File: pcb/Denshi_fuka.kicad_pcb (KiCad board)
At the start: 2 copper layers, 100 x 150 mm, 73 parts, among them J1 Power, J10 JST_PH2P, J11 JST_PH2P, J12 FAN_CONN1, J13 FAN_CONN2, J2 Analog, J3 Digital/PWM, J4 Digital/PWM, J5 SCREW TERMINAL, J6 SCREW TERMINAL, J7 SCREW TERMINAL, J8 SCREW TERMINAL, J9 SCREW TERMINAL, K2 SRD05VDCSLC, Q1 2SC1815, Q2 2SK3176, Q3 2SK3176, U1 Si8651, U10 MCP3564R, U2 LM2940T-3.3, U3 LM358, U4 MCP6232, U5 PS817, U6 PS817, U7 PS817, U8 PS817, U9 MCP4822

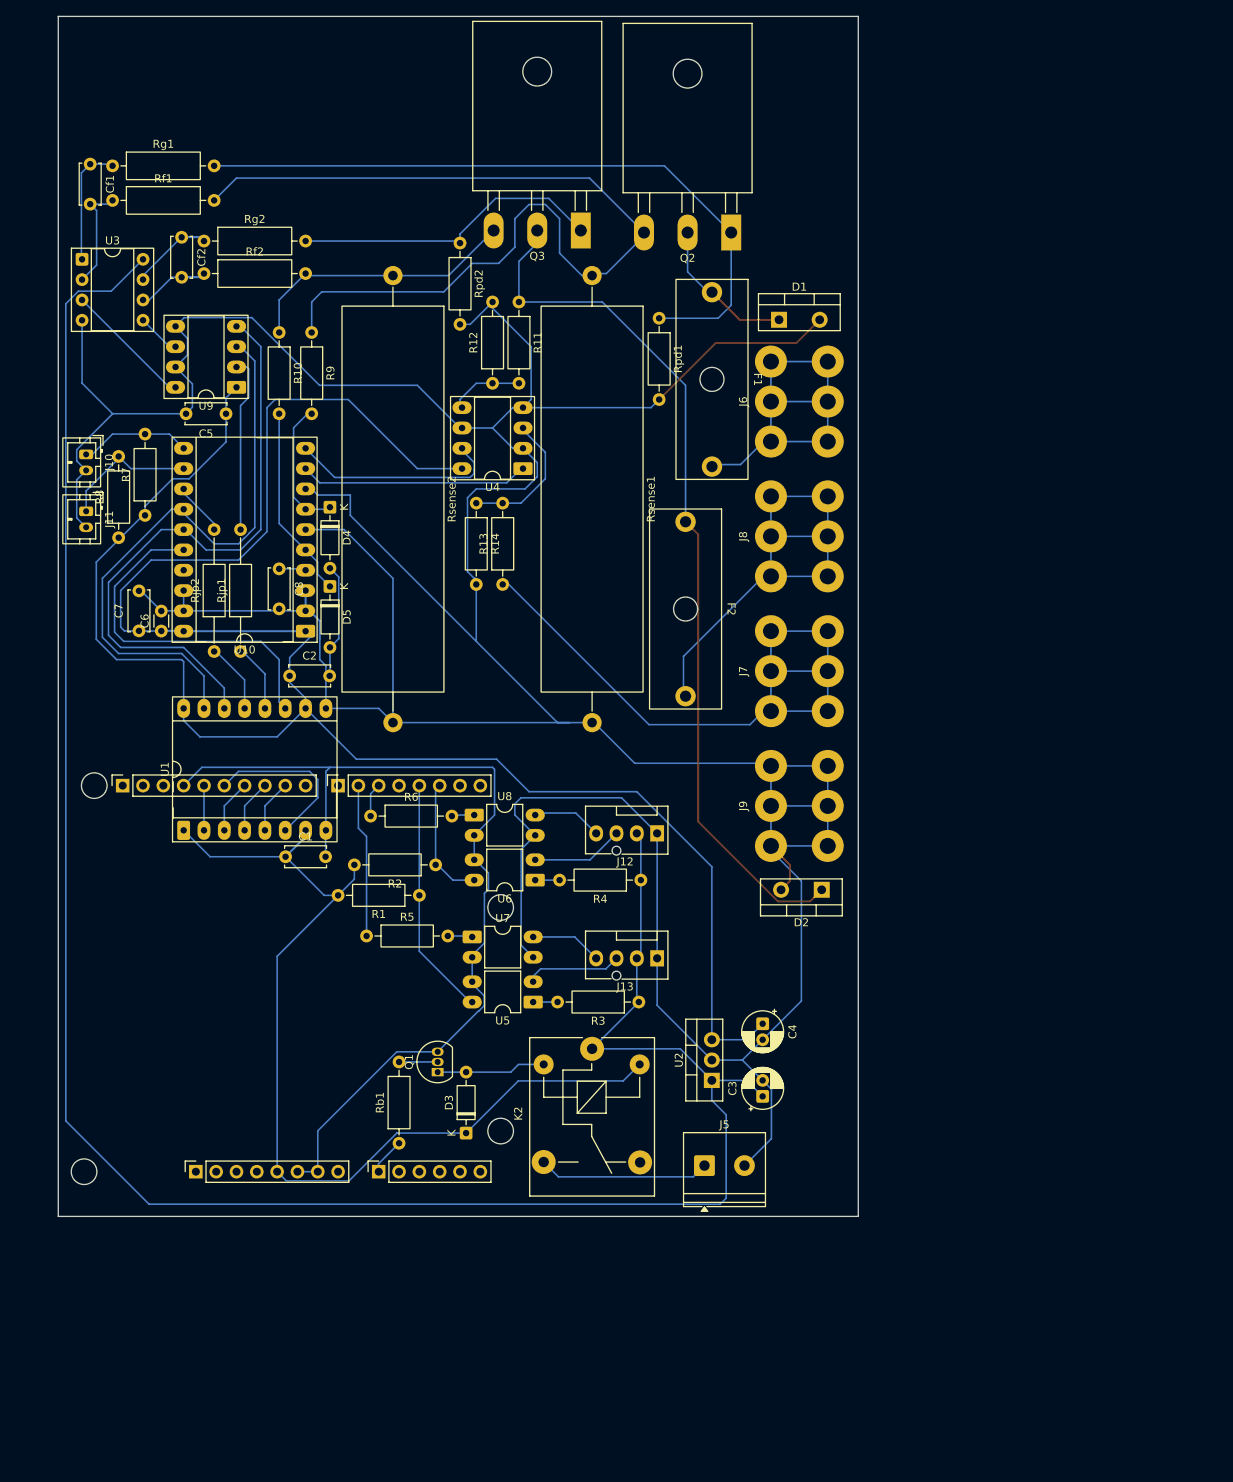
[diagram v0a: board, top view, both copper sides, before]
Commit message: pcb kansei
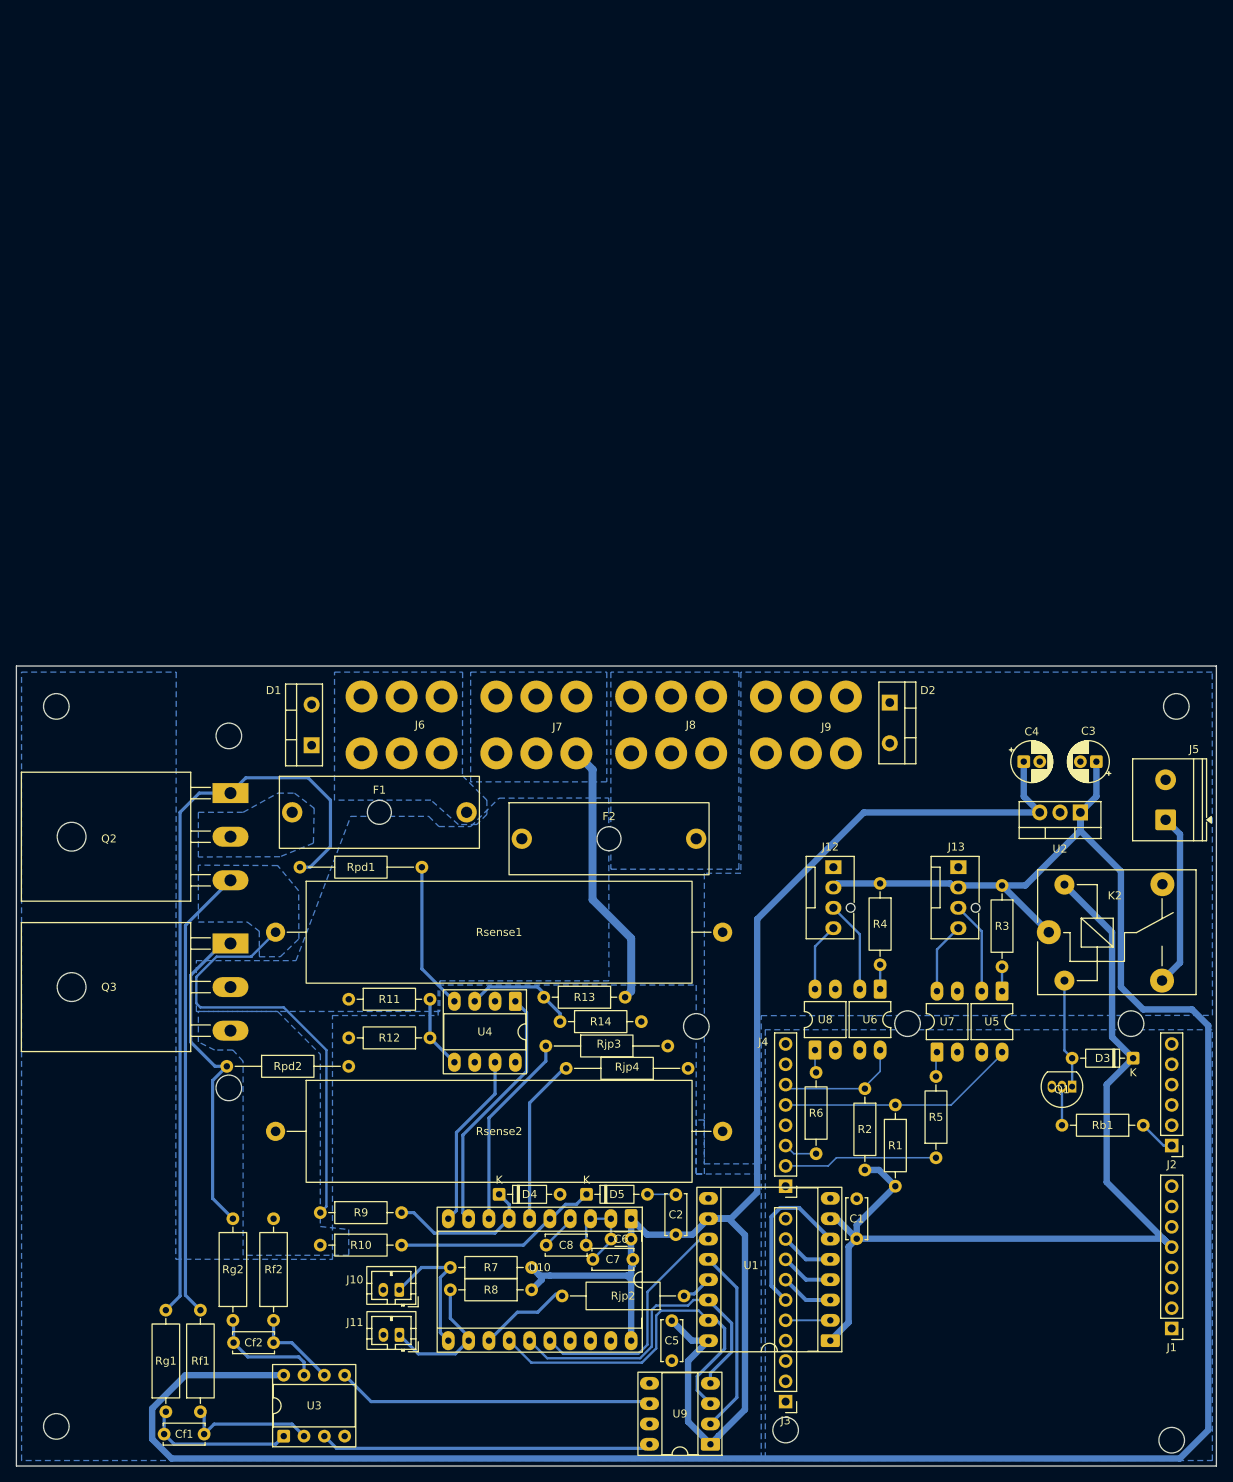
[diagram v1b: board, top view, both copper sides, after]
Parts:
- removed Rjp1: 0Ω, Resistor_THT:R_Axial_DIN0207_L6.3mm_D2.5mm_P15.24mm_Horizontal
- added ?: , , F.Cu at (110.5, 38.8)
- added ?: , , F.Cu at (188.5, 77.9)
- added ? (x2): , , F.Cu at (132.1, 42.9)
- added ?: , , F.Cu at (105.5, 130.1)
- added ?: , , F.Cu at (251.2, 38.6)
- added Rjp3: 0Ω, Resistor_THT:R_Axial_DIN0207_L6.3mm_D2.5mm_P15.24mm_Horizontal, F.Cu at (171.7, 81.7)
- added Rjp4: 0Ω, Resistor_THT:R_Axial_DIN0207_L6.3mm_D2.5mm_P15.24mm_Horizontal, F.Cu at (174.2, 84.5)
- J1: value Power -> Conn_01x08; footprint Connector_PinSocket_2.54mm:PinSocket_1x08_P2.54mm_Vertical -> Connector_PinHeader_2.54mm:PinHeader_1x08_P2.54mm_Vertical
- J2: value Analog -> Conn_01x06; footprint Connector_PinSocket_2.54mm:PinSocket_1x06_P2.54mm_Vertical -> Connector_PinHeader_2.54mm:PinHeader_1x06_P2.54mm_Vertical
- J3: value Digital/PWM -> Conn_01x10; footprint Connector_PinSocket_2.54mm:PinSocket_1x10_P2.54mm_Vertical -> Connector_PinHeader_2.54mm:PinHeader_1x10_P2.54mm_Vertical
- J4: value Digital/PWM -> Conn_01x08; footprint Connector_PinSocket_2.54mm:PinSocket_1x08_P2.54mm_Vertical -> Connector_PinHeader_2.54mm:PinHeader_1x08_P2.54mm_Vertical
- Rjp2: footprint Resistor_THT:R_Axial_DIN0207_L6.3mm_D2.5mm_P15.24mm_Horizontal -> Resistor_THT:R_Axial_DIN0309_L9.0mm_D3.2mm_P15.24mm_Horizontal
- Rpd1, Rpd2: footprint Resistor_THT:R_Axial_DIN0207_L6.3mm_D2.5mm_P10.16mm_Horizontal -> Resistor_THT:R_Axial_DIN0207_L6.3mm_D2.5mm_P15.24mm_Horizontal
- moved Cf1 159.0 mm to (124.0, 130.3), turned to 0 degrees
- moved Rg1 155.9 mm to (124.2, 127.5), turned to 90 degrees
- moved Rf1 151.8 mm to (128.5, 127.5), turned to 90 degrees
- moved U3 149.2 mm to (138.9, 130.5), turned to 90 degrees
- moved U9 144.8 mm to (192.3, 131.5)
- moved MH2 140.0 mm to (249.9, 131.0), turned to 90 degrees
- moved Cf2 138.3 mm to (132.7, 118.8), turned to 0 degrees
- moved Rg2 135.0 mm to (132.6, 116.0), turned to 90 degrees
- moved Rf2 131.1 mm to (137.7, 116.0), turned to 90 degrees
- moved C5 126.3 mm to (187.4, 116.1), turned to -90 degrees
- moved J1 123.5 mm to (249.9, 117.1), turned to 180 degrees
- moved MH1 118.1 mm to (201.7, 129.8), turned to 90 degrees
- moved R10 114.2 mm to (143.5, 106.6), turned to 0 degrees
- moved J3 113.1 mm to (201.7, 126.2), turned to 180 degrees
- moved J10 111.5 mm to (153.4, 112.2), turned to 180 degrees
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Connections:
- net Net-(J6-Pin_1) renamed /VDC1_IN
- net Net-(J8-Pin_1) renamed /VDC2_IN
- U10 pad 6: GNDA -> /ADC_i2-
- U10 pad 8: GNDA -> /ADC_i1-
- U9 pad 2: Net-(U9-~{CS}) -> /CS_MCP4822
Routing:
- net GNDA: track 567.3 -> 34.4 mm
- net GNDD: track 120.1 -> 0.00 mm
- net VDC2: track 110.6 -> 0.25 mm
- net +3V3_A: track 270.2 -> 186.0 mm
- net /VDC2_IN: track 60.7 -> 0.00 mm
- net /VDC1_IN: track 49.9 -> 0.00 mm
- net VDC1_Sense: track 82.4 -> 33.6 mm
- net /SDI: track 77.2 -> 41.7 mm
- net Net-(Q3-S): track 34.5 -> 0.00 mm
- net /Vout2: track 5.43 -> 39.6 mm
- net /SCK: track 75.6 -> 45.6 mm
- net +12V: track 270.0 -> 295.8 mm
- net /Vout1: track 16.2 -> 41.7 mm
- net /ADC_i1-: track 0.00 -> 24.5 mm
- net Net-(U9-~{CS}): track 22.1 -> 0.00 mm
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- added copper zone on B.Cu, net /VDC1_IN
- added copper zone on B.Cu, net /VDC2_IN
- added copper zone on B.Cu, net GNDA
- added copper zone on B.Cu, net GNDD
- added copper zone on B.Cu, net Net-(Q2-S)
- added copper zone on B.Cu, net Net-(Q3-S)
- added copper zone on B.Cu, net VDC1
- added copper zone on B.Cu, net VDC1_Sense
- added copper zone on B.Cu, net VDC2
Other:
- board size 100 x 150 mm -> 150 x 100 mm
